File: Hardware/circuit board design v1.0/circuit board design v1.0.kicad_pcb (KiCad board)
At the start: 4 copper layers, 30 x 80 mm, 47 parts, among them IC1 BMI088, J1 Conn_01x06_Male, J2 Conn_01x02, J3 105017-0001, J4 Conn_01x04, Q1 2N7002-7-F, U1 STM32F446RETx, U2 W25Q64JVSS, U3 SDR08540M3-01, U4 BME280, U5 STF202-22T1G, U6 MAX40203_SOT23, U7 NCP161ASN180T1G, U8 L80-R, Y1 Crystal_GND24

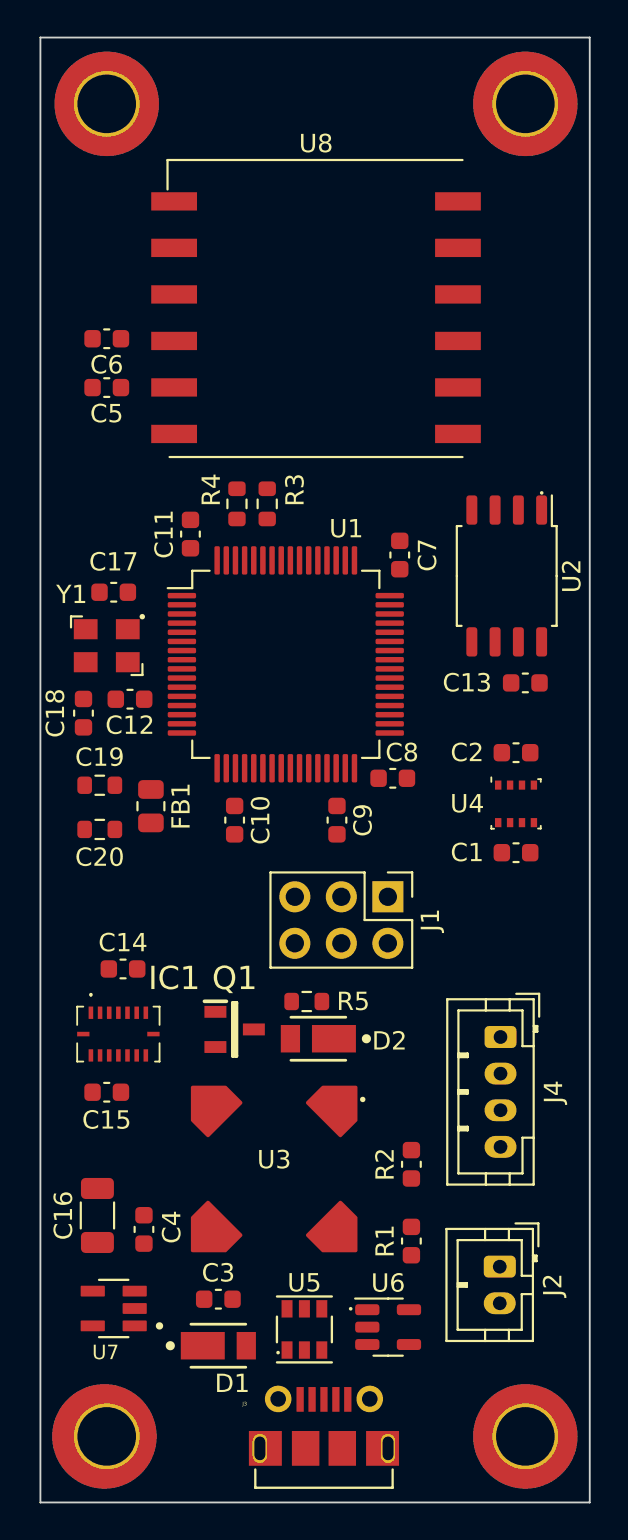
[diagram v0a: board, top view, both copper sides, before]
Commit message: Finished routing
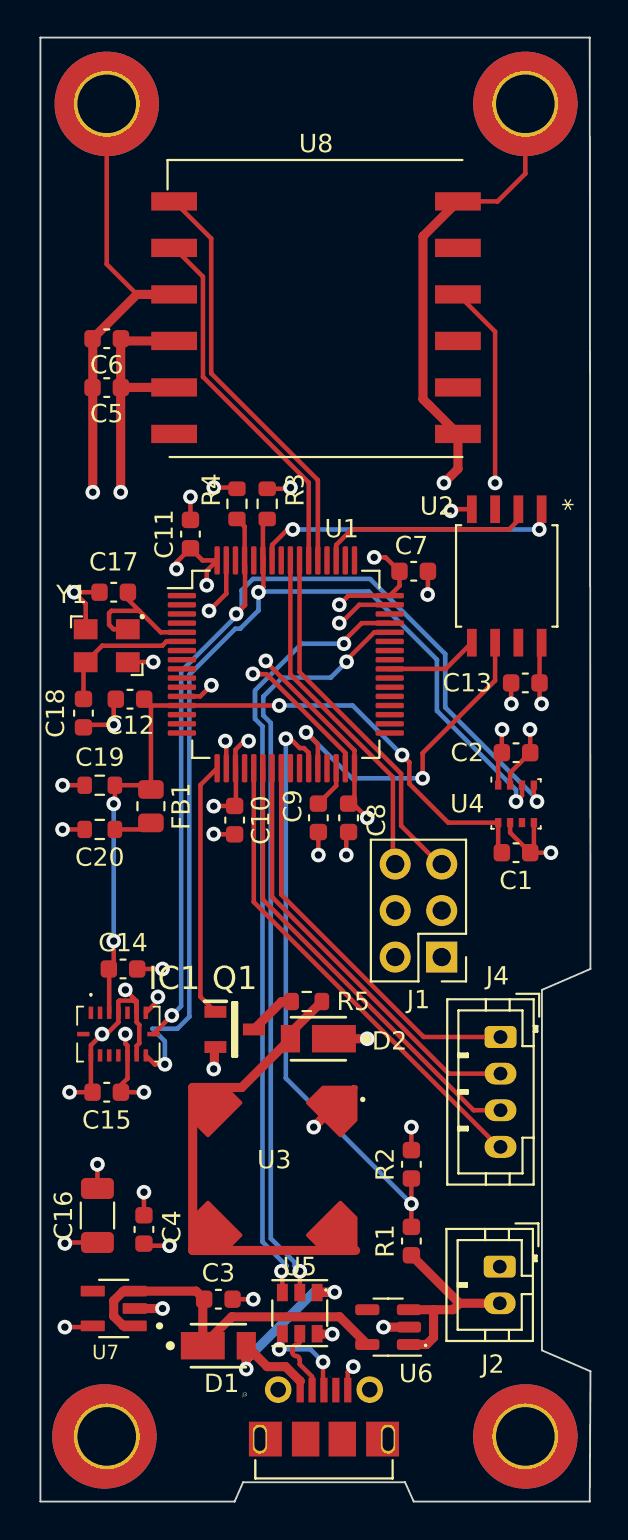
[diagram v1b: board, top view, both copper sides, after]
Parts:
- J2: footprint Connector_JST:JST_PH_B2B-PH-K_1x02_P2.00mm_Vertical -> Components:JST_PH_B2B-PH-K_1x02_P2.00mm_Vertical
- J4: footprint Connector_JST:JST_PH_B4B-PH-K_1x04_P2.00mm_Vertical -> Components:JST_PH_B4B-PH-K_1x04_P2.00mm_Vertical
- U1: footprint Package_QFP:LQFP-64_10x10mm_P0.5mm -> Components:LQFP-64_10x10mm_P0.5mm
- U2: footprint Package_SO:SOIC-8_5.23x5.23mm_P1.27mm -> Components:W25Q64JVSSIQ
- moved J1 4.41 mm to (41.9, 70.2), turned to 180 degrees
- moved C8 3.24 mm to (36.8, 62.6), turned to -90 degrees
- moved C7 1.17 mm to (40.4, 49.1), turned to 0 degrees
- moved C9 1.02 mm to (35.2, 62.6)
- moved U5 0.92 mm to (34.2, 89.7), turned to 180 degrees
- moved J3 0.51 mm to (35.5, 96.5)
- turned C2 to 180 degrees
- turned C20 to 180 degrees
- turned U6 to 180 degrees
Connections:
- U1 pad 25: /MCU/PWR_BVOLTS -> unconnected-(U1-Pad25)
- U1 pad 27: unconnected-(U1-Pad27) -> /MCU/PWR_BVOLTS
- U3 pad 2: GND -> Net-(D2-Pad2)
- U3 pad 3: GND -> Net-(D2-Pad2)
- U3 pad 4: GND -> Net-(D2-Pad2)
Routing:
- net GND: track 0.00 -> 120.9 mm, vias 0 -> 34
- net +3.3V: track 0.00 -> 77.7 mm, vias 0 -> 22
- net /MCU/SDA: track 0.00 -> 57.0 mm, vias 0 -> 3
- net /MCU/SCL: track 0.00 -> 55.7 mm, vias 0 -> 3
- net +3.3VA: track 0.00 -> 44.3 mm, vias 0 -> 4
- net /MCU/usb_dp: track 0.00 -> 42.7 mm, vias 0 -> 2
- net /MCU/usb_dm: track 0.00 -> 41.8 mm, vias 0 -> 2
- net /MCU/PWR_BVOLTS: track 0.00 -> 33.3 mm, vias 0 -> 2
- net Net-(D2-Pad2): track 0.00 -> 27.0 mm
- net /MCU/SPI1_SCK: track 0.00 -> 26.3 mm
- net /MCU/SPI1_MISO: track 0.00 -> 24.9 mm
- net /MCU/SPI1_MOSI: track 0.00 -> 23.5 mm
- net /GPS/rx_gps: track 0.00 -> 22.9 mm
- net /MCU/Radio_Enable: track 0.00 -> 22.1 mm
- net Net-(C3-Pad1): track 0.00 -> 20.4 mm
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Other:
- board size 30 x 80 mm -> 30 x 79.9 mm
